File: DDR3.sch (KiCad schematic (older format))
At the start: 31 parts, among them U11 W9751G6KB, U12 W9751G6KB, U5 xc7z020clg400

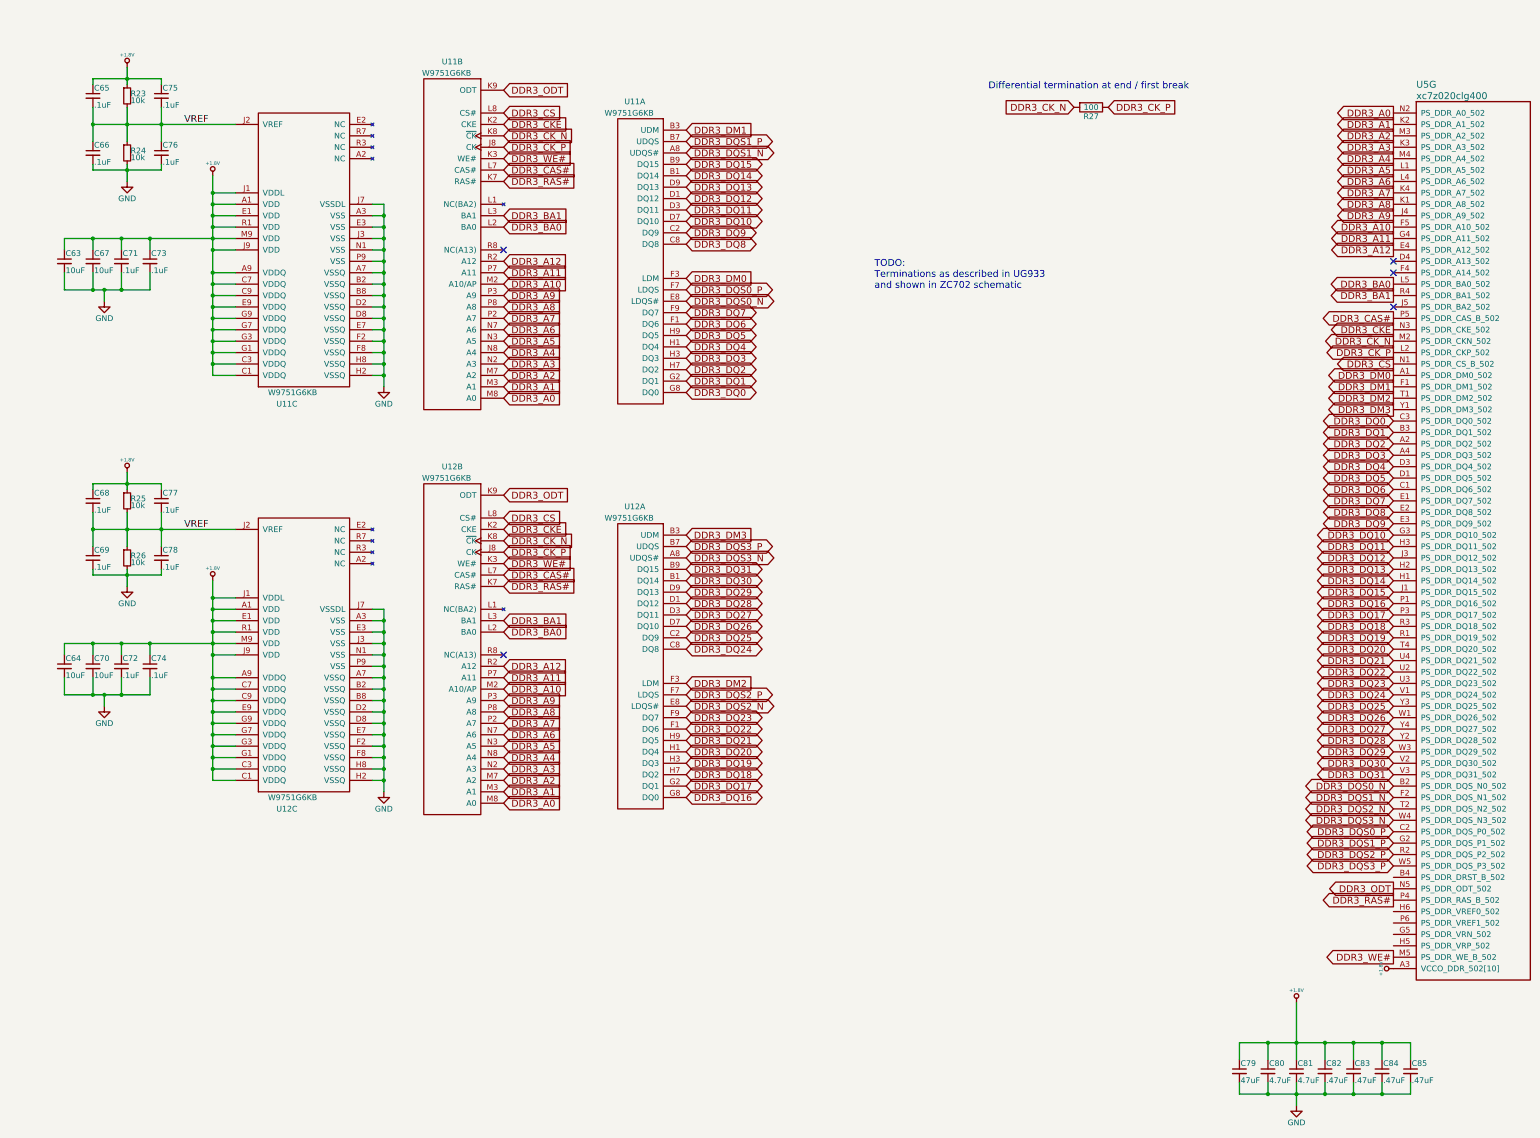
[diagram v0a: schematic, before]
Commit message: passes ERC, about to update footprints to v5 references
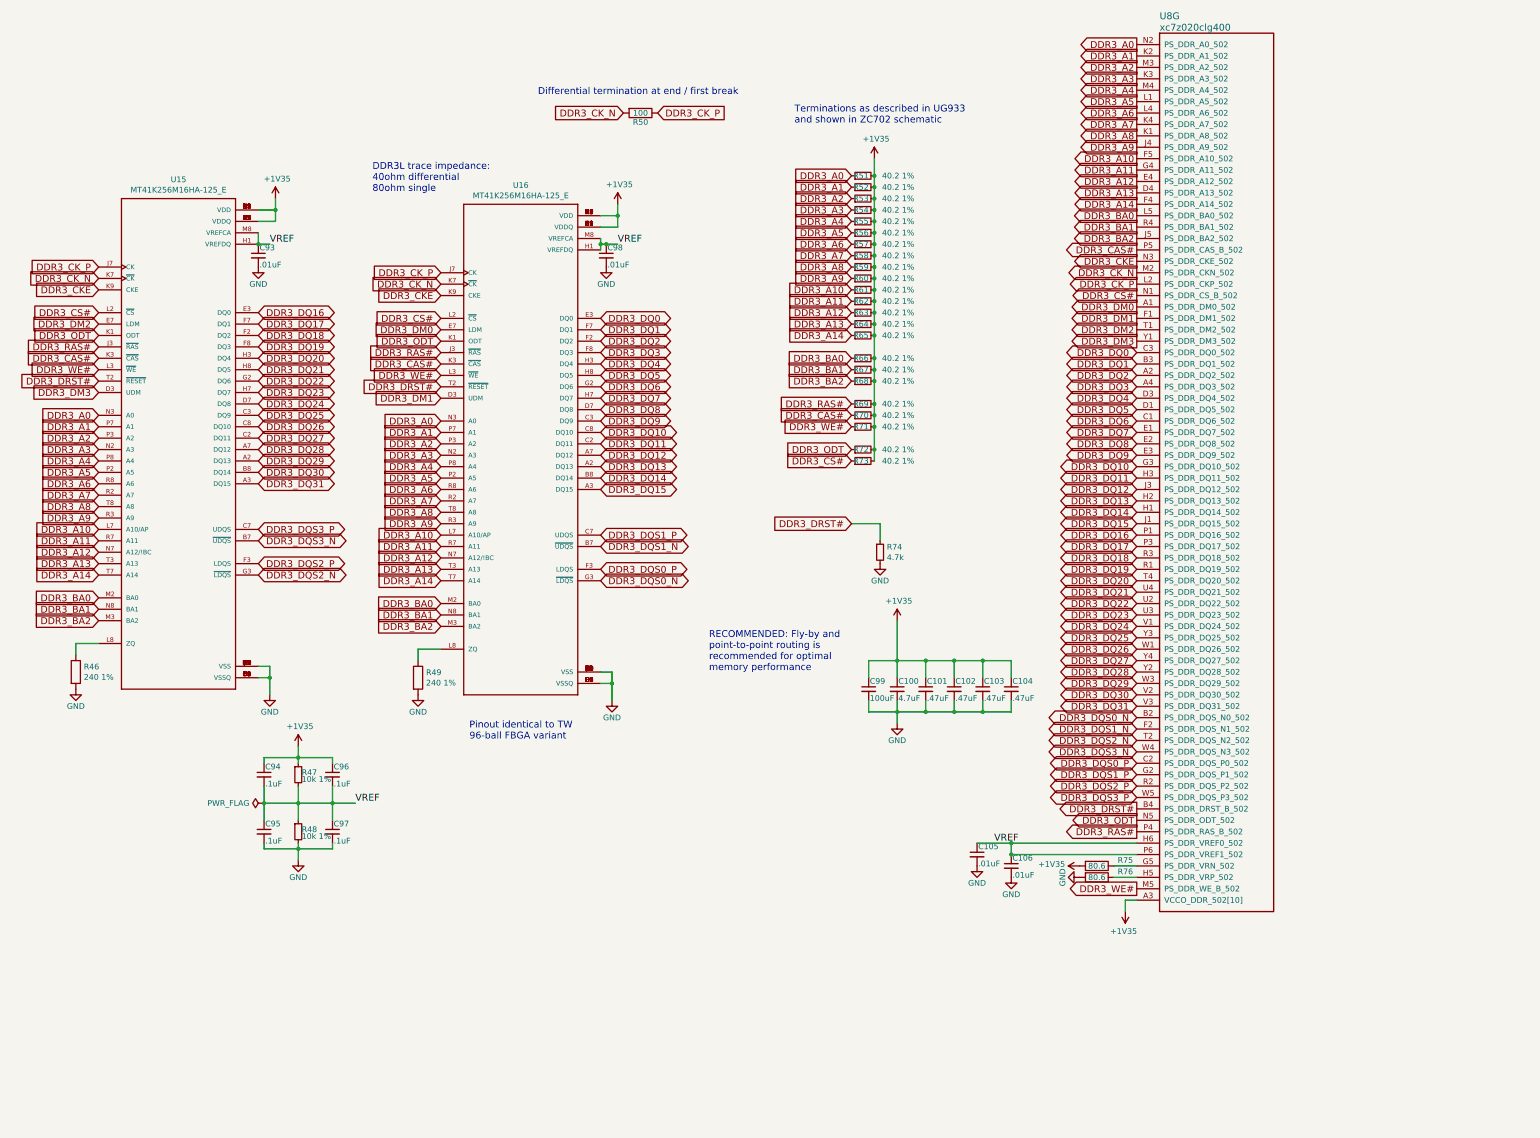
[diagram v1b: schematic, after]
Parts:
- removed C63, C64, C67, C70: 10uF, Capacitors_SMD:C_0603, symbol DFTBoard-rescue:C_Small-
- removed C68, C69, C71, C72, C73, C74, C77, C78: .1uF, Capacitors_SMD:C_0603, symbol DFTBoard-rescue:C_Small-
- removed C79: 47uF, Capacitors_SMD:C_1210, symbol DFTBoard-rescue:C_Small-
- removed C80: 4.7uF, Capacitors_SMD:C_0603, symbol DFTBoard-rescue:C_Small-
- removed R24, R25, R26: 10k, Resistors_SMD:R_0402, symbol DFTBoard-rescue:R_Small-
- removed U11, U12: W9751G6KB, DFTcustom:WBGA-84, symbol DFTBoard-rescue:W9751G6KB-
- added C105, C106, C93, C98: .01uF, Capacitors_SMD:C_0603, symbol DFTBoard-rescue:C_Small-
- added C99: 100uF, Capacitors_SMD:C_1210, symbol DFTBoard-rescue:C_Small-
- added R46, R49: 240 1%, Resistor_SMD:R_0402_1005Metric, symbol Device:R
- added R48: 10k 1%, Resistors_SMD:R_0402, symbol DFTBoard-rescue:R_Small-
- added R51, R52, R53, R54, R55, R56, R57, R58, R59, R60, R61, R62, R63, R64, R65, R66, R67, R68, R69, R70, R71, R72, R73: 40.2 1%, Resistor_SMD:R_0201_0603Metric, symbol DFTBoard-rescue:R_Small
- added R74: 4.7k, Resistor_SMD:R_0402_1005Metric, symbol DFTBoard-rescue:R_Small
- added R75, R76: 80.6, Resistor_SMD:R_0402_1005Metric, symbol Device:R
- added U15, U16: MT41K256M16HA-125_E, DFTcustom:FBGA-96-DDR3-SDRAM, symbol MT41K256M16HA-125_E:MT41K256M16HA-125_E
- R47: renamed from R23; value 10k -> 10k 1%; MPN RC0402FR-0710KL -> (none); SPN 311-10.0KLRTR-ND -> (none)
- U8: renamed from U5; footprint (none) -> Package_BGA:BGA-400_21.0x21.0mm_Layout20x20_P1.0mm
- renumbered C81 to C100, C82 to C101, C83 to C102, C84 to C103, C85 to C104, C65 to C94, C66 to C95, C75 to C96, C76 to C97, R27 to R50
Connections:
- net DDR3_A0: now also R51.1, U15.N3 (A0), U16.N3 (A0)
- net DDR3_A1: now also R52.1, U15.P7 (A1), U16.P7 (A1)
- net DDR3_A10: now also R61.1, U15.L7 (A10/AP), U16.L7 (A10/AP)
- net DDR3_A11: now also R62.1, U15.R7 (A11), U16.R7 (A11)
- net DDR3_A12: now also R63.1, U15.N7 (A12/!BC), U16.N7 (A12/!BC)
- net DDR3_A2: now also R53.1, U15.P3 (A2), U16.P3 (A2)
- net DDR3_A3: now also R54.1, U15.N2 (A3), U16.N2 (A3)
- net DDR3_A4: now also R55.1, U15.P8 (A4), U16.P8 (A4)
- net DDR3_A5: now also R56.1, U15.P2 (A5), U16.P2 (A5)
- net DDR3_A6: now also R57.1, U15.R8 (A6), U16.R8 (A6)
- net DDR3_A7: now also R58.1, U15.R2 (A7), U16.R2 (A7)
- net DDR3_A8: now also R59.1, U15.T8 (A8), U16.T8 (A8)
- net DDR3_A9: now also R60.1, U15.R3 (A9), U16.R3 (A9)
- net DDR3_BA0: now also R66.1, U15.M2 (BA0), U16.M2 (BA0)
- net DDR3_BA1: now also R67.1, U15.N8 (BA1), U16.N8 (BA1)
- net DDR3_CAS#: now also R70.1, U15.K3 (~CAS~), U16.K3 (~CAS~)
- net DDR3_CKE: now also U15.K9 (CKE), U16.K9 (CKE)
- net DDR3_CK_N: now also U15.K7 (~CK~), U16.K7 (~CK~)
- net DDR3_CK_P: now also U15.J7 (CK), U16.J7 (CK)
- net DDR3_DM0: now also U16.E7 (LDM)
- net DDR3_DM1: now also U16.D3 (UDM)
- net DDR3_DM2: now also U15.E7 (LDM)
- net DDR3_DM3: now also U15.D3 (UDM)
- net DDR3_DQ0: now also U16.E3 (DQ0)
- net DDR3_DQ1: now also U16.F7 (DQ1)
- net DDR3_DQ10: now also U16.C8 (DQ10)
- net DDR3_DQ11: now also U16.C2 (DQ11)
- net DDR3_DQ12: now also U16.A7 (DQ12)
- net DDR3_DQ13: now also U16.A2 (DQ13)
- net DDR3_DQ14: now also U16.B8 (DQ14)
- net DDR3_DQ15: now also U16.A3 (DQ15)
- net DDR3_DQ16: now also U15.E3 (DQ0)
- net DDR3_DQ17: now also U15.F7 (DQ1)
- net DDR3_DQ18: now also U15.F2 (DQ2)
- net DDR3_DQ19: now also U15.F8 (DQ3)
- net DDR3_DQ2: now also U16.F2 (DQ2)
- net DDR3_DQ20: now also U15.H3 (DQ4)
- net DDR3_DQ21: now also U15.H8 (DQ5)
- net DDR3_DQ22: now also U15.G2 (DQ6)
- net DDR3_DQ23: now also U15.H7 (DQ7)
- net DDR3_DQ24: now also U15.D7 (DQ8)
- net DDR3_DQ25: now also U15.C3 (DQ9)
- net DDR3_DQ26: now also U15.C8 (DQ10)
- net DDR3_DQ27: now also U15.C2 (DQ11)
- net DDR3_DQ28: now also U15.A7 (DQ12)
- net DDR3_DQ29: now also U15.A2 (DQ13)
- net DDR3_DQ3: now also U16.F8 (DQ3)
- net DDR3_DQ30: now also U15.B8 (DQ14)
- net DDR3_DQ31: now also U15.A3 (DQ15)
- net DDR3_DQ4: now also U16.H3 (DQ4)
- net DDR3_DQ5: now also U16.H8 (DQ5)
- net DDR3_DQ6: now also U16.G2 (DQ6)
- net DDR3_DQ7: now also U16.H7 (DQ7)
- net DDR3_DQ8: now also U16.D7 (DQ8)
- net DDR3_DQ9: now also U16.C3 (DQ9)
- net DDR3_DQS0_N: now also U16.G3 (~LDQS~)
- net DDR3_DQS0_P: now also U16.F3 (LDQS)
- net DDR3_DQS1_N: now also U16.B7 (~UDQS~)
- net DDR3_DQS1_P: now also U16.C7 (UDQS)
- net DDR3_DQS2_N: now also U15.G3 (~LDQS~)
- net DDR3_DQS2_P: now also U15.F3 (LDQS)
- net DDR3_DQS3_N: now also U15.B7 (~UDQS~)
- net DDR3_DQS3_P: now also U15.C7 (UDQS)
- net DDR3_ODT: now also R72.1, U15.K1 (ODT), U16.K1 (ODT)
- net DDR3_RAS#: now also R69.1, U15.J3 (~RAS~), U16.J3 (~RAS~)
- net DDR3_WE#: now also R71.1, U15.L3 (~WE~), U16.L3 (~WE~)
- net GND: now also C105.2, C106.2, C93.2, C98.2, C99.2, R46.2, R48.2, R49.2, R74.2, R76.2, U15.A9 (VSS), U15.B1 (VSSQ), U15.B3 (VSS), U15.B9 (VSSQ), U15.D1 (VSSQ), U15.D8 (VSSQ), U15.E1 (VSS), U15.E2 (VSSQ), U15.E8 (VSSQ), U15.F9 (VSSQ), U15.G1 (VSSQ), U15.G8 (VSS), U15.G9 (VSSQ), U15.J2 (VSS), U15.J8 (VSS), U15.M1 (VSS), U15.M9 (VSS), U15.P1 (VSS), U15.P9 (VSS), U15.T1 (VSS), U15.T9 (VSS), U16.A9 (VSS), U16.B1 (VSSQ), U16.B3 (VSS), U16.B9 (VSSQ), U16.D1 (VSSQ), U16.D8 (VSSQ), U16.E1 (VSS), U16.E2 (VSSQ), U16.E8 (VSSQ), U16.F9 (VSSQ), U16.G1 (VSSQ), U16.G8 (VSS), U16.G9 (VSSQ), U16.J2 (VSS), U16.J8 (VSS), U16.M1 (VSS), U16.M9 (VSS), U16.P1 (VSS), U16.P9 (VSS), U16.T1 (VSS), U16.T9 (VSS)
- net VREF: now also U8.H6 (PS_DDR_VREF0_502), U8.P6 (PS_DDR_VREF1_502), C105.1, C106.1, C93.1, C98.1, R48.1, U15.H1 (VREFDQ), U15.M8 (VREFCA), U16.H1 (VREFDQ), U16.M8 (VREFCA)
- net DDR3_DRST#: now reaches U8.B4 (PS_DDR_DRST_B_502)
- net DDR3_DRST#: now also R74.1, U15.T2 (~RESET~), U16.T2 (~RESET~)
- net DDR3_A13: now reaches U8.D4 (PS_DDR_A13_502)
- net DDR3_A13: now also R64.1, U15.T3 (A13), U16.T3 (A13)
- net DDR3_A14: now reaches U8.F4 (PS_DDR_A14_502)
- net DDR3_A14: now also R65.1, U15.T7 (A14), U16.T7 (A14)
- net at U8.G5 (PS_DDR_VRN_502): now also R75.1
- net at U8.H5 (PS_DDR_VRP_502): now also R76.1
- net DDR3_BA2: now reaches U8.J5 (PS_DDR_BA2_502)
- net DDR3_BA2: now also R68.1, U15.M3 (BA2), U16.M3 (BA2)
- net +1.8V renamed +1V35
- net +1V35: now also C99.1, R51.2, R52.2, R53.2, R54.2, R55.2, R56.2, R57.2, R58.2, R59.2, R60.2, R61.2, R62.2, R63.2, R64.2, R65.2, R66.2, R67.2, R68.2, R69.2, R70.2, R71.2, R72.2, R73.2, R75.2, U15.A1 (VDDQ), U15.A8 (VDDQ), U15.B2 (VDD), U15.C1 (VDDQ), U15.C9 (VDDQ), U15.D2 (VDDQ), U15.D9 (VDD), U15.E9 (VDDQ), U15.F1 (VDDQ), U15.G7 (VDD), U15.H2 (VDDQ), U15.H9 (VDDQ), U15.K2 (VDD), U15.K8 (VDD), U15.N1 (VDD), U15.N9 (VDD), U15.R1 (VDD), U15.R9 (VDD), U16.A1 (VDDQ), U16.A8 (VDDQ), U16.B2 (VDD), U16.C1 (VDDQ), U16.C9 (VDDQ), U16.D2 (VDDQ), U16.D9 (VDD), U16.E9 (VDDQ), U16.F1 (VDDQ), U16.G7 (VDD), U16.H2 (VDDQ), U16.H9 (VDDQ), U16.K2 (VDD), U16.K8 (VDD), U16.N1 (VDD), U16.N9 (VDD), U16.R1 (VDD), U16.R9 (VDD)
- net DDR3_CS renamed DDR3_CS#
- net DDR3_CS#: now also R73.1, U15.L2 (~CS~), U16.L2 (~CS~)
- new net: R49.1, U16.L8 (ZQ)
- new net: R46.1, U15.L8 (ZQ)
- no-connect marks 5 -> 0
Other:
- note added: "DDR3L trace impedance:\n40ohm differential\n80ohm single"
- note added: "Pinout identical to TW \n96-ball FBGA variant\n"
- note added: "RECOMMENDED: Fly-by and \npoint-to-point routing is\nrecommended for optimal \nmemory performance"
- note added: "Terminations as described in UG933\nand shown in ZC702 schematic"
- note removed: "TODO: \nTerminations as described in UG933\nand shown in ZC702 schematic"
- moved on the sheet: C100, C101, C102, C103, C104, C94, C95, C96, C97, R47, R50, U8G
